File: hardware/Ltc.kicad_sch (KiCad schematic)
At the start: 20 parts, among them IC1 LTC6804HG-1#PBF

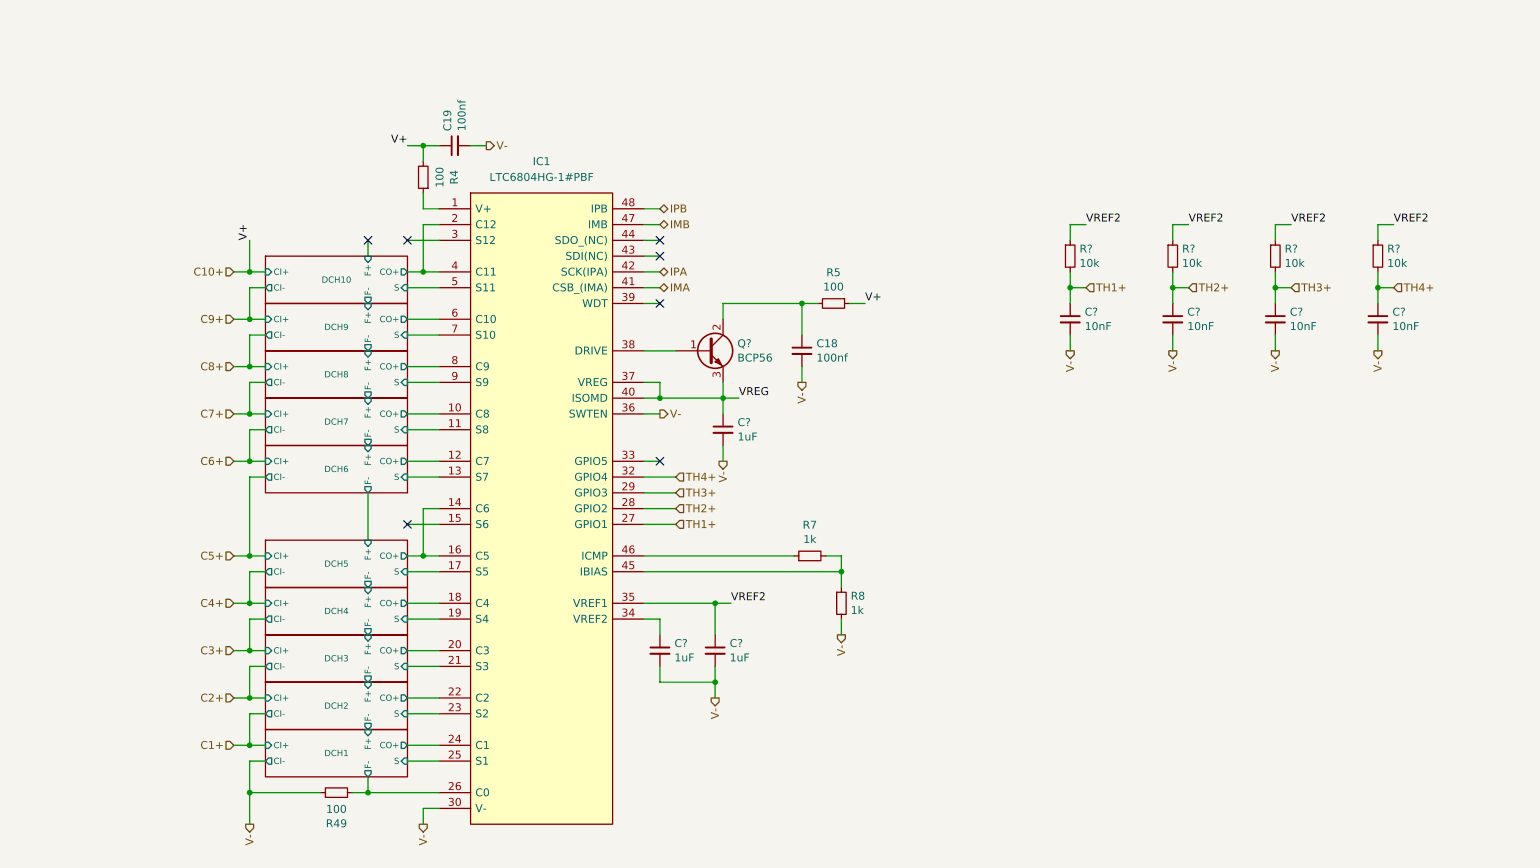
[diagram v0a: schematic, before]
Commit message: spaced out version
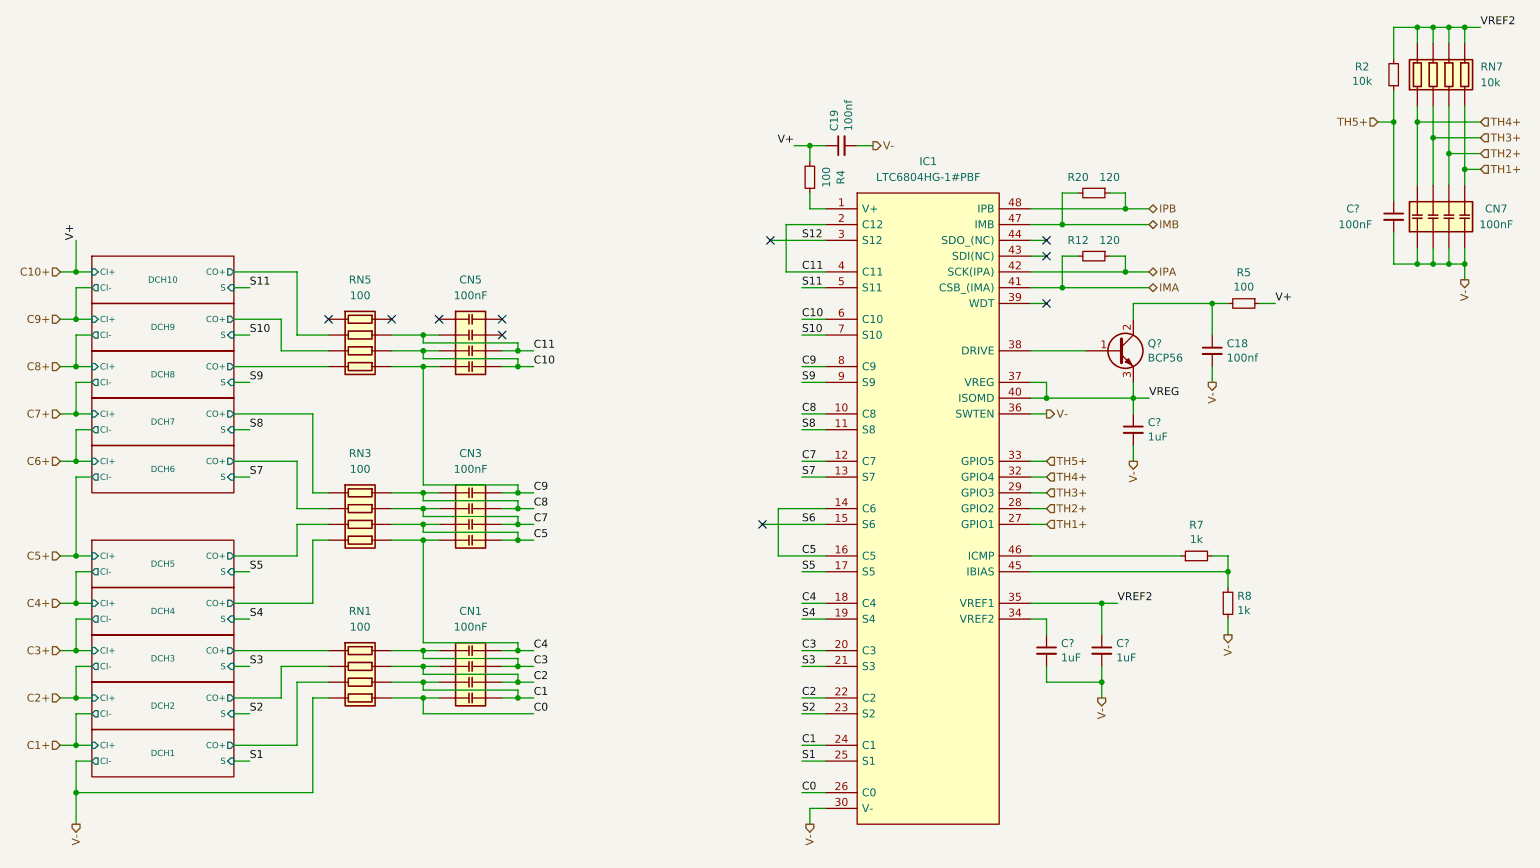
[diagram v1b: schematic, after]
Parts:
- removed C? (x4): 10nF, Capacitor_SMD:C_0603_1608Metric, symbol PUTM_EV_BMS_HV_Slave_2021-rescue:C_Small-Device
- removed R49: 100, Resistor_SMD:R_0603_1608Metric, symbol PUTM_EV_BMS_HV_Slave_2021-rescue:R_Small-Device
- removed R? (x4): 10k, Resistor_SMD:R_0603_1608Metric, symbol PUTM_EV_BMS_HV_Slave_2021-rescue:R_Small-Device
- added C?: 100nF, Capacitor_SMD:C_0603_1608Metric, symbol PUTM_EV_BMS_HV_Slave_2021-rescue:C_Small-Device
- added CN1, CN3, CN5, CN7: 100nF, Samacsys:CA064X104K4RACAUTO, symbol ca064x104k4racauto:CA064X104K4RACAUTO
- added R12, R20: 120, Resistor_SMD:R_0603_1608Metric, symbol PUTM_EV_BMS_HV_Slave_2021-rescue:R_Small-Device
- added R2: 10k, Resistor_SMD:R_0603_1608Metric, symbol PUTM_EV_BMS_HV_Slave_2021-rescue:R_Small-Device
- added RN1, RN3, RN5: 100, Samacsys:EXBV8V101JV, symbol exb-v8v101jv:EXB-V8V101JV
- added RN7: 10k, Samacsys:EXBV8V101JV, symbol exb-v8v101jv:EXB-V8V101JV
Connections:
- net DCH1/CO+: now also RN1.3 (R3.1); no longer IC1.24 (C1)
- net DCH10/CO+: now also RN5.2 (R2.1); no longer IC1.2 (C12), IC1.4 (C11)
- net DCH2/CO+: now also RN1.2 (R2.1); no longer IC1.22 (C2)
- net DCH3/CO+: now also RN1.1 (R1.1); no longer IC1.20 (C3)
- net DCH4/CO+: now also RN3.4 (R4.1); no longer IC1.18 (C4)
- net DCH5/CO+: now also RN3.3 (R3.1); no longer IC1.14 (C6), IC1.16 (C5)
- net DCH6/CO+: now also RN3.2 (R2.1); no longer IC1.12 (C7)
- net DCH7/CO+: now also RN3.1 (R1.1); no longer IC1.10 (C8)
- net DCH8/CO+: now also RN5.4 (R4.1); no longer IC1.8 (C9)
- net DCH9/CO+: now also RN5.3 (R3.1); no longer IC1.6 (C10)
- net IMA: now also R12.2
- net IMB: now also R20.2
- net IPA: now also R12.1
- net IPB: now also R20.1
- net TH1+: now also CN7.5 (R4.2), RN7.4 (R4.1)
- net TH2+: now also CN7.6 (R3.2), RN7.3 (R3.1)
- net TH3+: now also CN7.7 (R2.2), RN7.2 (R2.1)
- net TH4+: now also CN7.8 (R1.2), RN7.1 (R1.1)
- net V-: now also C?.2, CN7.1 (R1.1), CN7.2 (R2.1), CN7.3 (R3.1), CN7.4 (R4.1), RN1.4 (R4.1)
- net VREF2: now also R2.2, RN7.5 (R4.2), RN7.6 (R3.2), RN7.7 (R2.2), RN7.8 (R1.2)
- net S6: now reaches IC1.15 (S6)
- net S12: now reaches IC1.3 (S12)
- net TH5+: now reaches IC1.33 (GPIO5)
- net TH5+: now also C?.1, R2.1
- net DCH1/F- renamed C0
- net C0: now also CN1.4 (R4.1), RN1.5 (R4.2)
- net DCH1/S renamed S1
- net DCH10/S renamed S11
- net DCH2/S renamed S2
- net DCH3/S renamed S3
- net DCH4/S renamed S4
- net DCH5/S renamed S5
- net DCH6/S renamed S7
- net DCH7/S renamed S8
- net DCH8/S renamed S9
- net DCH9/S renamed S10
- new net C1: CN1.3 (R3.1), CN1.5 (R4.2), IC1.24 (C1), RN1.6 (R3.2)
- new net C10: CN5.3 (R3.1), CN5.5 (R4.2), IC1.6 (C10), RN5.6 (R3.2)
- new net C11: CN5.2 (R2.1), CN5.6 (R3.2), IC1.2 (C12), IC1.4 (C11), RN5.7 (R2.2)
- new net C2: CN1.2 (R2.1), CN1.6 (R3.2), IC1.22 (C2), RN1.7 (R2.2)
- new net C3: CN1.1 (R1.1), CN1.7 (R2.2), IC1.20 (C3), RN1.8 (R1.2)
- new net C4: CN1.8 (R1.2), CN3.4 (R4.1), IC1.18 (C4), RN3.5 (R4.2)
- new net C5: CN3.3 (R3.1), CN3.5 (R4.2), IC1.14 (C6), IC1.16 (C5), RN3.6 (R3.2)
- new net C7: CN3.2 (R2.1), CN3.6 (R3.2), IC1.12 (C7), RN3.7 (R2.2)
- new net C8: CN3.1 (R1.1), CN3.7 (R2.2), IC1.10 (C8), RN3.8 (R1.2)
- new net C9: CN3.8 (R1.2), CN5.4 (R4.1), IC1.8 (C9), RN5.5 (R4.2)
- no-connect marks 7 -> 10
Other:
- sheet DCH1 ports: added none; removed F+, F-
- sheet DCH10 ports: added none; removed F+, F-
- sheet DCH2 ports: added none; removed F+, F-
- sheet DCH3 ports: added none; removed F+, F-
- sheet DCH4 ports: added none; removed F+, F-
- sheet DCH5 ports: added none; removed F+, F-
- sheet DCH6 ports: added none; removed F+, F-
- sheet DCH7 ports: added none; removed F+, F-
- sheet DCH8 ports: added none; removed F+, F-
- sheet DCH9 ports: added none; removed F+, F-
- moved on the sheet: C18, C19, C?, IC1, Q?, R4, R5, R7, R8
